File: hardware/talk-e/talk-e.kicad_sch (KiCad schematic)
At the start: 35 parts, among them J3 Conn_02x04_Odd_Even, J4 Conn_Coaxial, Q1 FS8205A, SW4 SS-12D00-G 4 E, SW5 SW_Push, U2 DW01A, U3 TP4056-42-ESOP8, U5 AP2112K-3.3

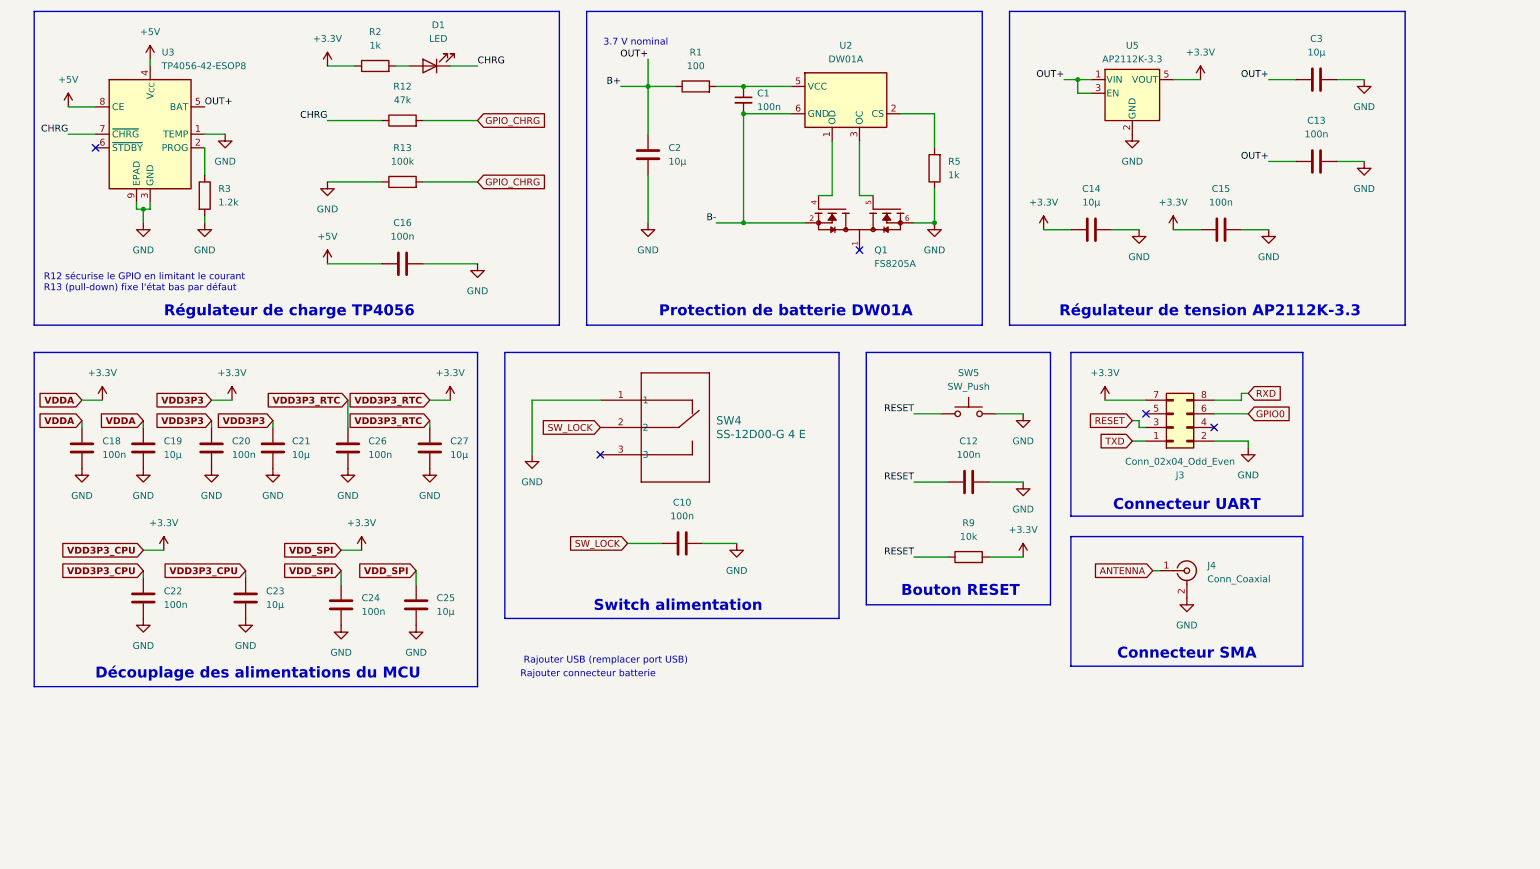
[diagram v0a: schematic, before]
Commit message: Finished routing + PCB ready for production
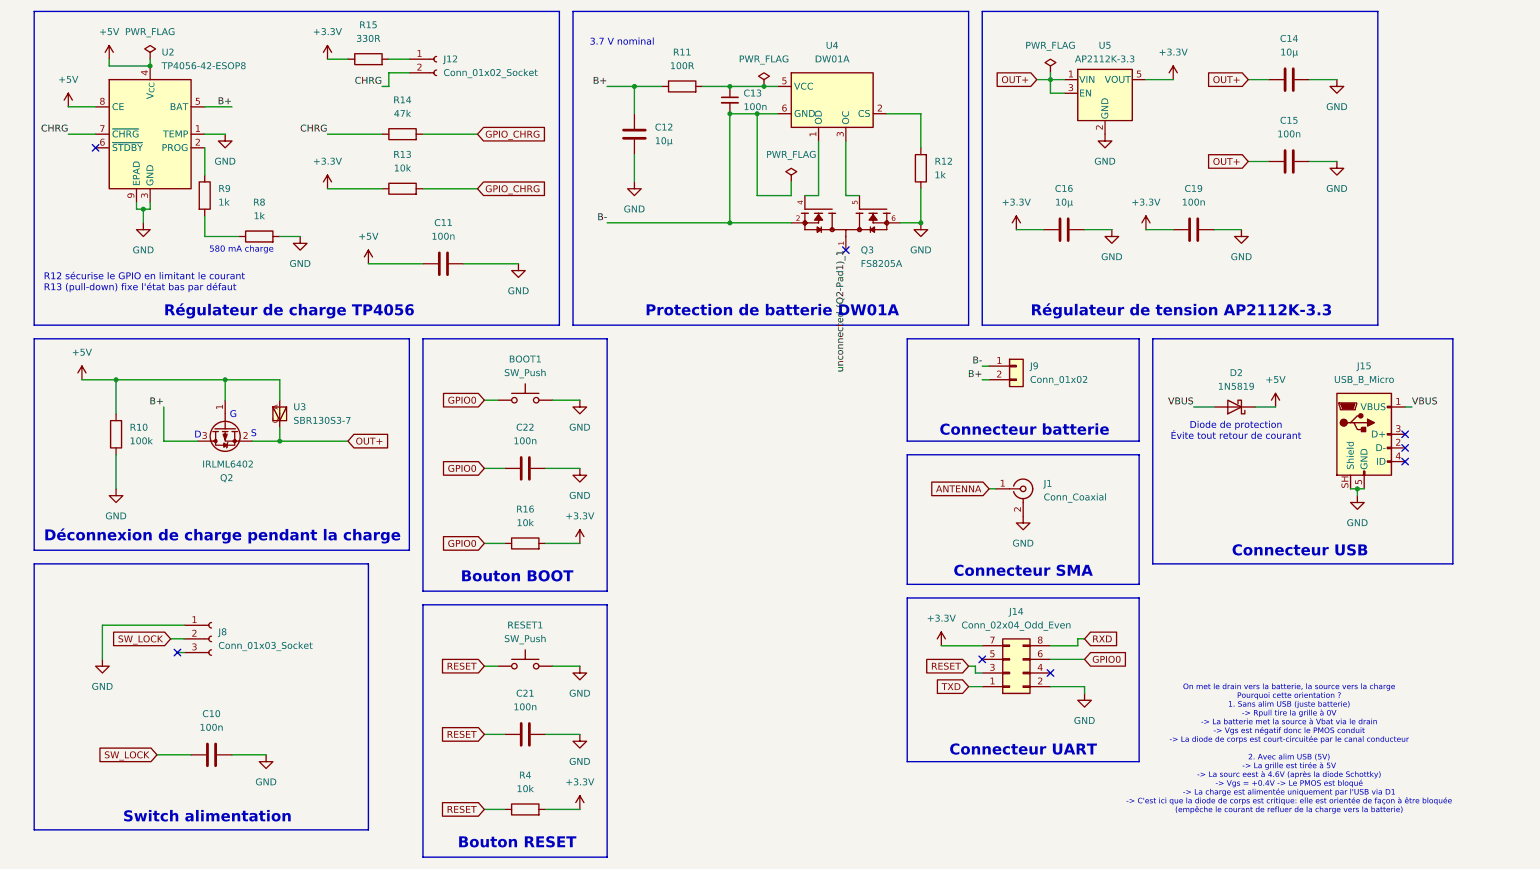
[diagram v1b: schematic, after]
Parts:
- removed C18, C20, C24, C26: 100n, symbol Device:C
- removed C19, C21, C23, C25, C27: 10µ, symbol Device:C
- removed D1: LED, LED_THT:LED_D3.0mm, symbol Device:LED
- removed J3: Conn_02x04_Odd_Even, Connector_IDC:IDC-Header_2x04_P2.54mm_Vertical, symbol Connector_Generic:Conn_02x04_Odd_Even
- removed R2: 1k, symbol Device:R
- removed SW4: SS-12D00-G 4 E, 1P2T_SS-12D00_CNK, symbol 2026-05-09_16-09-49:SS-12D00-G_4_E
- added BOOT1: SW_Push, Button_Switch_THT:SW_PUSH_6mm, symbol Switch:SW_Push
- added D2: 1N5819, Diode_THT:D_DO-41_SOD81_P10.16mm_Horizontal, symbol Diode:1N5819
- added J12: Conn_01x02_Socket, Connector_JST:JST_EH_B2B-EH-A_1x02_P2.50mm_Vertical, symbol Connector:Conn_01x02_Socket
- added J14: Conn_02x04_Odd_Even, Connector_PinHeader_2.54mm:PinHeader_2x04_P2.54mm_Horizontal, symbol Connector_Generic:Conn_02x04_Odd_Even
- added J15: USB_B_Micro, Connector_USB:USB_Micro-AB_Molex_47590-0001, symbol Connector:USB_B_Micro
- added J8: Conn_01x03_Socket, Connector_JST:JST_EH_B3B-EH-A_1x03_P2.50mm_Vertical, symbol Connector:Conn_01x03_Socket
- added J9: Conn_01x02, Connector_JST:JST_EH_B2B-EH-A_1x02_P2.50mm_Vertical, symbol Connector_Generic:Conn_01x02
- added Q2: IRLML6402, Package_TO_SOT_SMD:SOT-23, symbol Transistor_FET:IRLML6402
- added R10: 100k, Resistor_SMD:R_1206_3216Metric, symbol Device:R
- added R15: 330R, Resistor_SMD:R_1206_3216Metric, symbol Device:R
- added R16: 10k, Resistor_SMD:R_1206_3216Metric, symbol Device:R
- added R8: 1k, Resistor_SMD:R_1206_3216Metric, symbol Device:R
- added U3: SBR130S3-7, SBR130S3-7:SBR130S3-7, symbol SBR130S3-7:SBR130S3-7
- C10, C22: footprint (none) -> Capacitor_SMD:C_0805_2012Metric; KiLib_Generator (none) -> SMD_2terminal_chip_molded
- C11: renamed from C16; footprint (none) -> Capacitor_SMD:C_0805_2012Metric; KiLib_Generator (none) -> SMD_2terminal_chip_molded
- C12: renamed from C2; footprint (none) -> Capacitor_SMD:C_0805_2012Metric; KiLib_Generator (none) -> SMD_2terminal_chip_molded
- C13: renamed from C1; footprint (none) -> Capacitor_SMD:C_0805_2012Metric; KiLib_Generator (none) -> SMD_2terminal_chip_molded
- C14: renamed from C3; footprint (none) -> Capacitor_SMD:C_0805_2012Metric; KiLib_Generator (none) -> SMD_2terminal_chip_molded
- C15: renamed from C13; footprint (none) -> Capacitor_SMD:C_0805_2012Metric; KiLib_Generator (none) -> SMD_2terminal_chip_molded
- C16: renamed from C14; footprint (none) -> Capacitor_SMD:C_0805_2012Metric; KiLib_Generator (none) -> SMD_2terminal_chip_molded
- C19: renamed from C15; footprint (none) -> Capacitor_SMD:C_0805_2012Metric; KiLib_Generator (none) -> SMD_2terminal_chip_molded
- C21: renamed from C12; footprint (none) -> Capacitor_SMD:C_0805_2012Metric; KiLib_Generator (none) -> SMD_2terminal_chip_molded
- R11: renamed from R1; value 100 -> 100R; footprint (none) -> Resistor_SMD:R_1206_3216Metric; KiLib_Generator (none) -> SMD_2terminal_chip_molded
- R12: renamed from R5; footprint (none) -> Resistor_SMD:R_1206_3216Metric; KiLib_Generator (none) -> SMD_2terminal_chip_molded
- R13: value 100k -> 10k; footprint (none) -> Resistor_SMD:R_1206_3216Metric; KiLib_Generator (none) -> SMD_2terminal_chip_molded
- R14: renamed from R12; footprint (none) -> Resistor_SMD:R_1206_3216Metric; KiLib_Generator (none) -> SMD_2terminal_chip_molded
- R4: renamed from R9; footprint (none) -> Resistor_SMD:R_1206_3216Metric; KiLib_Generator (none) -> SMD_2terminal_chip_molded
- R9: renamed from R3; value 1.2k -> 1k; footprint (none) -> Resistor_SMD:R_1206_3216Metric; KiLib_Generator (none) -> SMD_2terminal_chip_molded
- RESET1: renamed from SW5; footprint (none) -> Button_Switch_THT:SW_PUSH_6mm
- U2: renamed from U3; KiLib_Generator (none) -> package/gullwing
- U4: renamed from U2; KiLib_Generator (none) -> package/gullwing
- U5: KiLib_Generator (none) -> package/gullwing
- renumbered J4 to J1, Q1 to Q3
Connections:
- net +3.3V: now also R13.1, J14.7 (Pin_7), R15.1, R16.2; no longer C22.2
- net +5V: now also D2.1 (K), Q2.1 (G), R10.2, U3.A
- net B+: now also J9.2 (Pin_2), Q2.3 (D); no longer C14.1, C15.1, U5.1 (VIN), U5.3 (EN)
- net B-: now also J9.1 (Pin_1)
- net CHRG: now also J12.2 (Pin_2)
- net GND: now also C22.2, BOOT1.2, J14.2 (Pin_2), J15.5 (GND), J15.SH (Shield), J8.1 (Pin_1), R10.1, R8.2; no longer C22.1, R13.1, R9.2
- net GPIO0: now also C22.1, BOOT1.1, J14.6 (Pin_6), R16.1
- net RESET: now also J14.3 (Pin_3)
- net RXD: now also J14.8 (Pin_8)
- net SW_LOCK: now also J8.2 (Pin_2)
- net TXD: now also J14.1 (Pin_1)
- net unconnected-(Q2-Pad1)_1: now reaches Q3.1, Q3.8
- new net: J12.1 (Pin_1), R15.2
- new net: R8.1, R9.2
- new net OUT+: C14.1, C15.1, Q2.2 (S), U3.C, U5.1 (VIN), U5.3 (EN)
- new net VBUS: D2.2 (A), J15.1 (VBUS)
- no-connect marks 5 -> 8
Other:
- note added: "580 mA charge"
- note added: "Bouton BOOT"
- note added: "Connecteur USB"
- note added: "Connecteur batterie"
- note added: "D"
- note added: "Diode de protection Évite tout retour de courant"
- note added: "Déconnexion de charge pendant la charge"
- note added: "G"
- note added: "On met le drain vers la batterie, la source vers la charge Pourquoi cette orientation ? 1. Sans alim USB (juste batterie) -> Rpull tire la grille à 0V -> La batterie met la source à Vbat via le drain -> Vgs est négatif donc le PMOS conduit -> La diode de corps est court-circuitée par le canal conducteur 2. Avec alim USB (5V) -> La grille est tirée à 5V -> La sourc eest à 4.6V (après la diode Scho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"
- note added: "S"
- note removed: "Découplage des alimentations du MCU"
- note removed: "Rajouter USB (remplacer port USB)"
- note removed: "Rajouter connecteur batterie"
- moved on the sheet: C10, C11, C12, C13, C14, C15, C16, C19, C21, J1, Q3, R11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
